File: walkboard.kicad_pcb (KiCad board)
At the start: 2 copper layers, 154 parts, among them J1 USB_C_Receptacle_USB2.0, SW1 SW_Push, U1 ATmega32U4-AU, Y1 Crystal_GND24_Small

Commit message: fixed
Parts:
- added BT1: Battery_Cell, Connector_JST:JST_XH_S2B-XH-A_1x02_P2.50mm_Horizontal, B.Cu at (258.9, 12.4)
- added C10: 4.7uF, Capacitor_SMD:C_0805_2012Metric_Pad1.15x1.40mm_HandSolder, B.Cu at (260.4, 48.8)
- added C11: 1uF, Capacitor_SMD:C_0805_2012Metric_Pad1.15x1.40mm_HandSolder, B.Cu at (256.2, 48.8)
- added C12: 22uF, Capacitor_SMD:C_0805_2012Metric_Pad1.15x1.40mm_HandSolder, B.Cu at (266.3, 57.1)
- added C8: C_Small, Capacitor_SMD:C_0805_2012Metric_Pad1.15x1.40mm_HandSolder, B.Cu at (255.6, 27.3)
- added C9: C_Small, Capacitor_SMD:C_0805_2012Metric_Pad1.15x1.40mm_HandSolder, B.Cu at (262.8, 21.4)
- added D69: D_Schottky, Diode_SMD:D_SOD-123, B.Cu at (253.8, 32.1)
- added L1: L_Small, Inductor_SMD:L_0805_2012Metric_Pad1.15x1.40mm_HandSolder, B.Cu at (259.8, 32.7)
- added Q1: Q_PMOS_DGS, Package_TO_SOT_SMD:SOT-23, B.Cu at (259.8, 28.5)
- added R10: R_Small, Resistor_SMD:R_0805_2012Metric_Pad1.15x1.40mm_HandSolder, B.Cu at (251.6, 37.4)
- added R7: 10K, Resistor_SMD:R_0805_2012Metric_Pad1.15x1.40mm_HandSolder, B.Cu at (250.3, 31.5)
- added R8: R_Small, Resistor_SMD:R_0805_2012Metric_Pad1.15x1.40mm_HandSolder, B.Cu at (258.5, 17.4)
- added R9: R_Small, Resistor_SMD:R_0805_2012Metric_Pad1.15x1.40mm_HandSolder, B.Cu at (258.0, 37.4)
- added U2: MCP73831-2-OT, Package_TO_SOT_SMD:SOT-23-5, B.Cu at (258.5, 21.2)
- added U3: TPS61200DRC, Package_SON:Texas_S-PVSON-N10_ThermalVias, B.Cu at (258.6, 42.8)
- C1, C2, C3, C4, C5, C6, D10, D11, D12, D13, D14, D17, D18, D19, D20, D21, D22, D23, D24, D25, D26, D27, D28, D30, D31, D32, D33, D34, D35, D36, D37, D38, D39, D4, D40, D41, D42, D43, D44, D45, D46, D47, D48, D49, D5, D50, D51, D52, D53, D54, D55, D56, D57, D58, D59, D6, D60, D61, D62, D63, D64, D65, D66, D67, D68, D7, D8, D9, J1, SW1, U1, Y1: moved to B.Cu
- C7: value 0.1uF -> 10uF; footprint Diode_SMD:D_SOD-123 -> Capacitor_SMD:C_0805_2012Metric_Pad1.15x1.40mm_HandSolder; moved to B.Cu
- F1: value 500mA -> Polyfuse_Small; footprint keyswitches:Kailh_socket_MX -> Fuse:Fuse_1206_3216Metric_Pad1.42x1.75mm_HandSolder; moved to B.Cu
- MX68: footprint Resistor_SMD:R_0805_2012Metric -> keyswitches:Kailh_socket_MX
- R1, R2, R3, R4: footprint Resistor_SMD:R_0612_1632Metric_Pad1.18x3.40mm_HandSolder -> Resistor_SMD:R_0805_2012Metric_Pad1.15x1.40mm_HandSolder; moved to B.Cu
- R5, R6: value 10k -> 5.1k; footprint Resistor_SMD:R_0612_1632Metric_Pad1.18x3.40mm_HandSolder -> Resistor_SMD:R_0805_2012Metric_Pad1.15x1.40mm_HandSolder; moved to B.Cu
- moved MX67 295.9 mm to (247.3, 85.1)
- moved MX56 286.4 mm to (271.1, 66.0)
- moved D56 277.7 mm to (276.8, 70.8), turned to 90 degrees
- moved MX66 274.3 mm to (228.2, 85.1)
- moved MX63 264.9 mm to (161.5, 85.1)
- moved MX65 258.3 mm to (209.2, 85.1)
- moved MX42 253.7 mm to (271.1, 47.0)
- moved MX64 247.8 mm to (190.1, 85.1)
- moved MX43 227.7 mm to (13.9, 66.0)
- moved R2 227.4 mm to (25.3, 9.82), turned to 90 degrees
- moved MX55 224.5 mm to (247.3, 66.0)
- moved MX41 222.1 mm to (247.3, 47.0)
- moved MX58 220.4 mm to (37.7, 85.1)
- moved D67 216.6 mm to (239.7, 89.8), turned to 90 degrees
- moved D55 216.4 mm to (239.7, 71.7), turned to 90 degrees
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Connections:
- C4 pad 1: +5V -> Net-(C12-Pad1)
- C4 pad 2: GND -> +5V
- C5 pad 1: +5V -> Net-(C12-Pad1)
- C5 pad 2: GND -> +5V
- C6 pad 1: +5V -> Net-(C12-Pad1)
- C6 pad 2: GND -> +5V
- C7 pad 1: +5V -> Net-(C12-Pad1)
- C7 pad 2: GND -> +5V
- F1 pad 1: +5V -> Net-(F1-Pad1)
- F1 pad 2: VCC -> Net-(C8-Pad1)
- J1 pad A4: VCC -> Net-(F1-Pad1)
- J1 pad A8: Net-(J1-PadA8) -> (no net)
- J1 pad A9: VCC -> Net-(F1-Pad1)
- J1 pad B4: VCC -> Net-(F1-Pad1)
- J1 pad B8: Net-(J1-PadB8) -> (no net)
- J1 pad B9: VCC -> Net-(F1-Pad1)
- U1 pad 1: Net-(U1-Pad1) -> (no net)
- U1 pad 10: Net-(U1-Pad10) -> (no net)
- U1 pad 11: Net-(U1-Pad11) -> (no net)
- U1 pad 12: Net-(U1-Pad12) -> (no net)
- U1 pad 18: Net-(U1-Pad18) -> (no net)
- U1 pad 19: Net-(U1-Pad19) -> (no net)
- U1 pad 20: Net-(U1-Pad20) -> (no net)
- U1 pad 21: Net-(U1-Pad21) -> (no net)
- U1 pad 22: Net-(U1-Pad22) -> (no net)
- U1 pad 25: Net-(U1-Pad25) -> (no net)
- U1 pad 26: Net-(U1-Pad26) -> (no net)
- U1 pad 27: Net-(U1-Pad27) -> (no net)
- U1 pad 28: Net-(U1-Pad28) -> (no net)
- U1 pad 29: Net-(U1-Pad29) -> (no net)
- U1 pad 30: Net-(U1-Pad30) -> (no net)
- U1 pad 31: Net-(U1-Pad31) -> (no net)
- U1 pad 32: Net-(U1-Pad32) -> (no net)
- U1 pad 36: Net-(U1-Pad36) -> (no net)
- U1 pad 37: Net-(U1-Pad37) -> (no net)
- U1 pad 38: Net-(U1-Pad38) -> (no net)
- U1 pad 39: Net-(U1-Pad39) -> (no net)
- U1 pad 40: Net-(U1-Pad40) -> (no net)
- U1 pad 41: Net-(U1-Pad41) -> (no net)
- U1 pad 42: Net-(U1-Pad42) -> (no net)
- U1 pad 8: Net-(U1-Pad8) -> (no net)
- U1 pad 9: Net-(U1-Pad9) -> (no net)
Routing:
- net ROW3: track 0.00 -> 273.9 mm, vias 0 -> 2
- net ROW2: track 0.00 -> 270.8 mm, vias 0 -> 2
- net ROW4: track 0.00 -> 263.2 mm, vias 0 -> 2
- net ROW1: track 0.00 -> 259.7 mm, vias 0 -> 2
- net ROW0: track 0.00 -> 244.1 mm, vias 0 -> 2
- net GND: track 0.00 -> 186.0 mm, vias 0 -> 20
- net COL7: track 0.00 -> 88.5 mm, vias 0 -> 8
- net COL5: track 0.00 -> 87.5 mm, vias 0 -> 8
- net COL1: track 0.00 -> 86.3 mm, vias 0 -> 8
- net COL3: track 0.00 -> 86.0 mm, vias 0 -> 8
- net COL12: track 0.00 -> 85.9 mm, vias 0 -> 7
- net COL4: track 0.00 -> 85.4 mm, vias 0 -> 9
- net COL10: track 0.00 -> 85.1 mm, vias 0 -> 8
- net COL9: track 0.00 -> 84.5 mm, vias 0 -> 8
- net COL11: track 0.00 -> 84.0 mm, vias 0 -> 8
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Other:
- board outline added: 285.4 x 94 mm
- net class Default: trace_width 0.25 -> 0.254
- net class Power added: clearance 0.2, trace_width 0.381, via_dia 0.8, via_drill 0.4

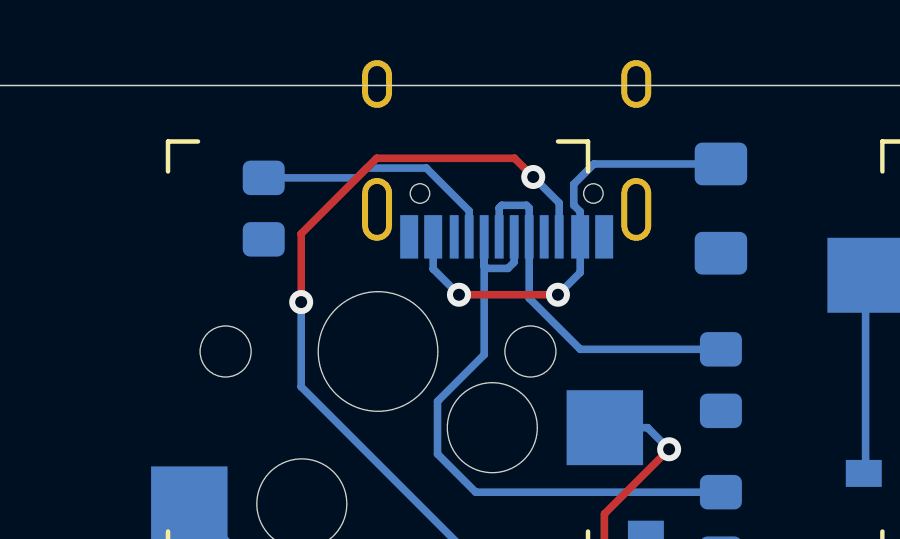
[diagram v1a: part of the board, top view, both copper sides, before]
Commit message: added stuff
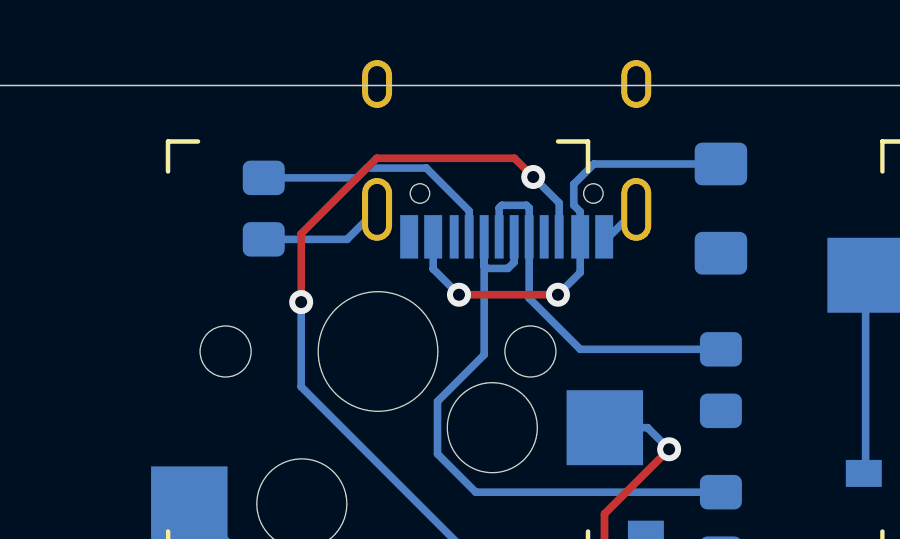
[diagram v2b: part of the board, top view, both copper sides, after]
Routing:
- net GND: track 186.0 -> 191.6 mm
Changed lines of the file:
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@@
     (thickness 1.6)
     (drawings 4)
-    (tracks 918)
+    (tracks 922)
     (zones 0)
     (modules 169)
@@
   (segment (start 254.545 48.118263) (end 256.203903 49.777166) (width 0.254) (layer B.Cu) (net 1))
   (segment (start 254.545 46.615) (end 254.545 48.118263) (width 0.254) (layer B.Cu) (net 1))
+  (segment (start 12.881321 5.128679) (end 13.88 4.13) (width 0.254) (layer B.Cu) (net 1))
+  (segment (start 10.101492 5.128679) (end 12.881321 5.128679) (width 0.254) (layer B.Cu) (net 1))
+  (segment (start 21.605 5.045) (end 22.52 4.13) (width 0.254) (layer B.Cu) (net 1))
+  (segment (start 21.45 5.045) (end 21.605 5.045) (width 0.254) (layer B.Cu) (net 1))
   (segment (start 256.369529 86.586572) (end 256.294529 86.511572) (width 0.254) (layer B.Cu) (net 2))
   (segment (start 256.369529 89.828763) (end 256.369529 86.586572) (width 0.254) (layer B.Cu) (net 2))
